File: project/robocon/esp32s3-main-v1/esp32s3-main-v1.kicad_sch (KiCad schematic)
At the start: 1 part, among them U1 ESP32-S3-WROOM-1

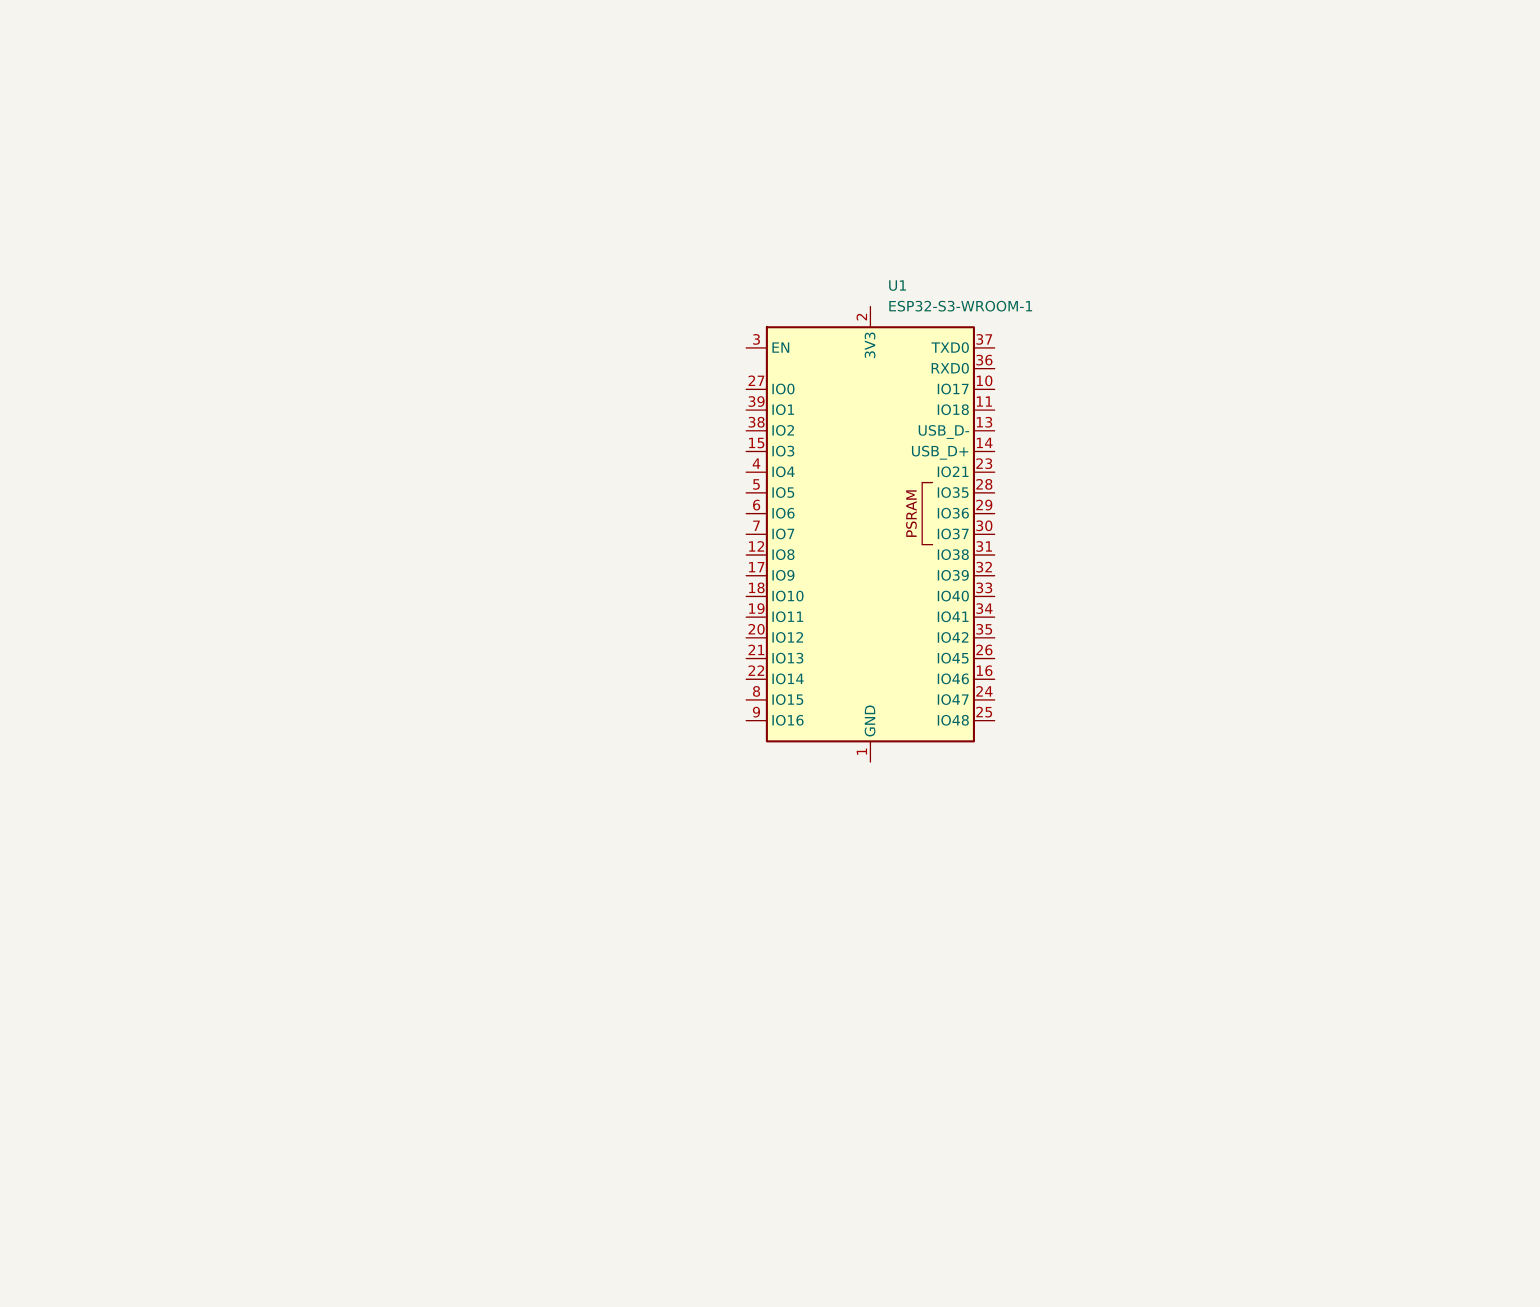
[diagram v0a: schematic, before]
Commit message: 2026/07/16/09:30
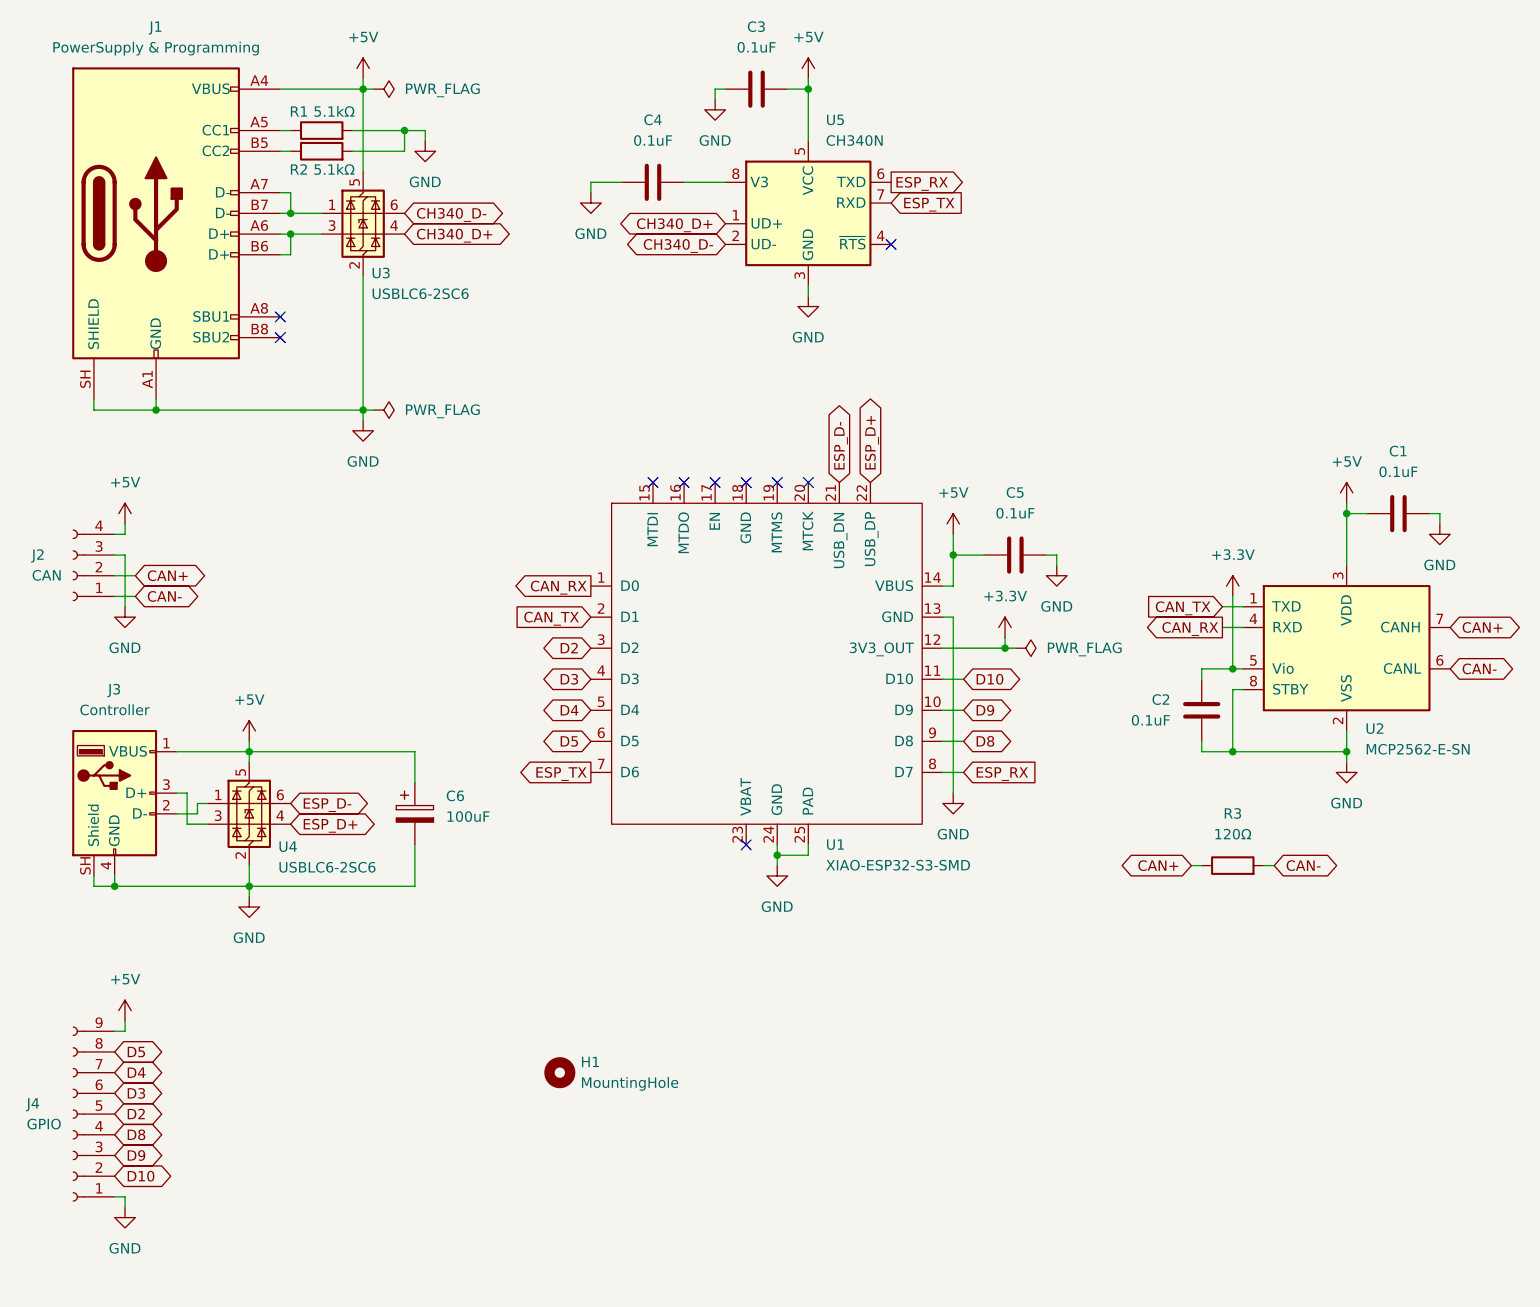
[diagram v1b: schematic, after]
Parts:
- removed U1: ESP32-S3-WROOM-1, RF_Module:ESP32-S3-WROOM-1, symbol RF_Module:ESP32-S3-WROOM-1
- added C1, C2, C3, C4, C5: 0.1uF, Capacitor_SMD:C_0603_1608Metric, symbol Device:C
- added C6: 100uF, Capacitor_THT:CP_Radial_D6.3mm_P2.50mm, symbol Device:C_Polarized
- added H1: MountingHole, MountingHole:MountingHole_3.2mm_M3, symbol Mechanical:MountingHole
- added J1: PowerSupply & Programming, Connector_USB:USB_C_Receptacle_GCT_USB4105-xx-A_16P_TopMnt_Horizontal, symbol Connector:USB_C_Receptacle_USB2.0_16P
- added J2: CAN, Connector_JST:JST_XH_S4B-XH-A_1x04_P2.50mm_Horizontal, symbol Connector:Conn_01x04_Socket
- added J3: Controller, Connector_USB:USB_A_Molex_67643_Horizontal, symbol Connector:USB_A
- added J4: GPIO, Connector_JST:JST_XH_B9B-XH-A_1x09_P2.50mm_Vertical, symbol Connector:Conn_01x09_Socket
- added R1, R2: 5.1kΩ, Resistor_SMD:R_0603_1608Metric, symbol Device:R
- added R3: 120Ω, Resistor_SMD:R_0603_1608Metric, symbol Device:R
- added U1: XIAO-ESP32-S3-SMD, Seeed Studio XIAO Series Library:XIAO-ESP32-S3-SMD, symbol Seeed_Studio_XIAO_Series:XIAO-ESP32-S3-SMD
- added U2: MCP2562-E-SN, Package_SO:SOIC-8_3.9x4.9mm_P1.27mm, symbol Interface_CAN_LIN:MCP2562-E-SN
- added U3, U4: USBLC6-2SC6, Package_TO_SOT_SMD:SOT-23-6, symbol Power_Protection:USBLC6-2SC6
- added U5: CH340N, Package_SO:JEITA_SOIC-8_3.9x4.9mm_P1.27mm, symbol Interface_USB:CH340N
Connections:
- new net: C4.1, U5.8 (V3)
- new net: J1.B5 (CC2), R2.1
- new net: J1.A5 (CC1), R1.1
- new net: J1.A7 (D-), J1.B7 (D-), U3.1 (I/O1)
- new net: J1.A6 (D+), J1.B6 (D+), U3.3 (I/O2)
- new net: J3.2 (D-), U4.1 (I/O1)
- new net: J3.3 (D+), U4.3 (I/O2)
- new net +3.3V: C2.1, U1.12 (3V3_OUT), U2.5 (Vio)
- new net +5V: C1.1, C3.1, C5.1, C6.1, J1.A4 (VBUS), J1.A9 (VBUS), J1.B4 (VBUS), J1.B9 (VBUS), J2.4 (Pin_4), J3.1 (VBUS), J4.9 (Pin_9), U1.14 (VBUS), U2.3 (VDD), U3.5 (VBUS), U4.5 (VBUS), U5.5 (VCC)
- new net CAN+: J2.2 (Pin_2), R3.1, U2.7 (CANH)
- new net CAN-: J2.1 (Pin_1), R3.2, U2.6 (CANL)
- new net CAN_RX: U1.1 (D0), U2.4 (RXD)
- new net CAN_TX: U1.2 (D1), U2.1 (TXD)
- new net CH340_D+: U3.4 (I/O2), U5.1 (UD+)
- new net CH340_D-: U3.6 (I/O1), U5.2 (UD-)
- new net D10: J4.2 (Pin_2), U1.11 (D10)
- new net D2: J4.5 (Pin_5), U1.3 (D2)
- new net D3: J4.6 (Pin_6), U1.4 (D3)
- new net D4: J4.7 (Pin_7), U1.5 (D4)
- new net D5: J4.8 (Pin_8), U1.6 (D5)
- new net D8: J4.4 (Pin_4), U1.9 (D8)
- new net D9: J4.3 (Pin_3), U1.10 (D9)
- new net ESP_D+: U1.22 (USB_DP), U4.4 (I/O2)
- new net ESP_D-: U1.21 (USB_DN), U4.6 (I/O1)
- new net ESP_RX: U1.8 (D7), U5.6 (TXD)
- new net ESP_TX: U1.7 (D6), U5.7 (RXD)
- new net GND: C1.2, C2.2, C3.2, C4.2, C5.2, C6.2, J1.A1 (GND), J1.A12 (GND), J1.B1 (GND), J1.B12 (GND), J1.SH (SHIELD), J2.3 (Pin_3), J3.4 (GND), J3.SH (Shield), J4.1 (Pin_1), R1.2, R2.2, U1.13 (GND), U1.24 (GND), U1.25 (PAD), U2.2 (VSS), U2.8 (STBY), U3.2 (GND), U4.2 (GND), U5.3 (GND)
- no-connect marks 0 -> 10

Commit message: 2026/07/16/16:32
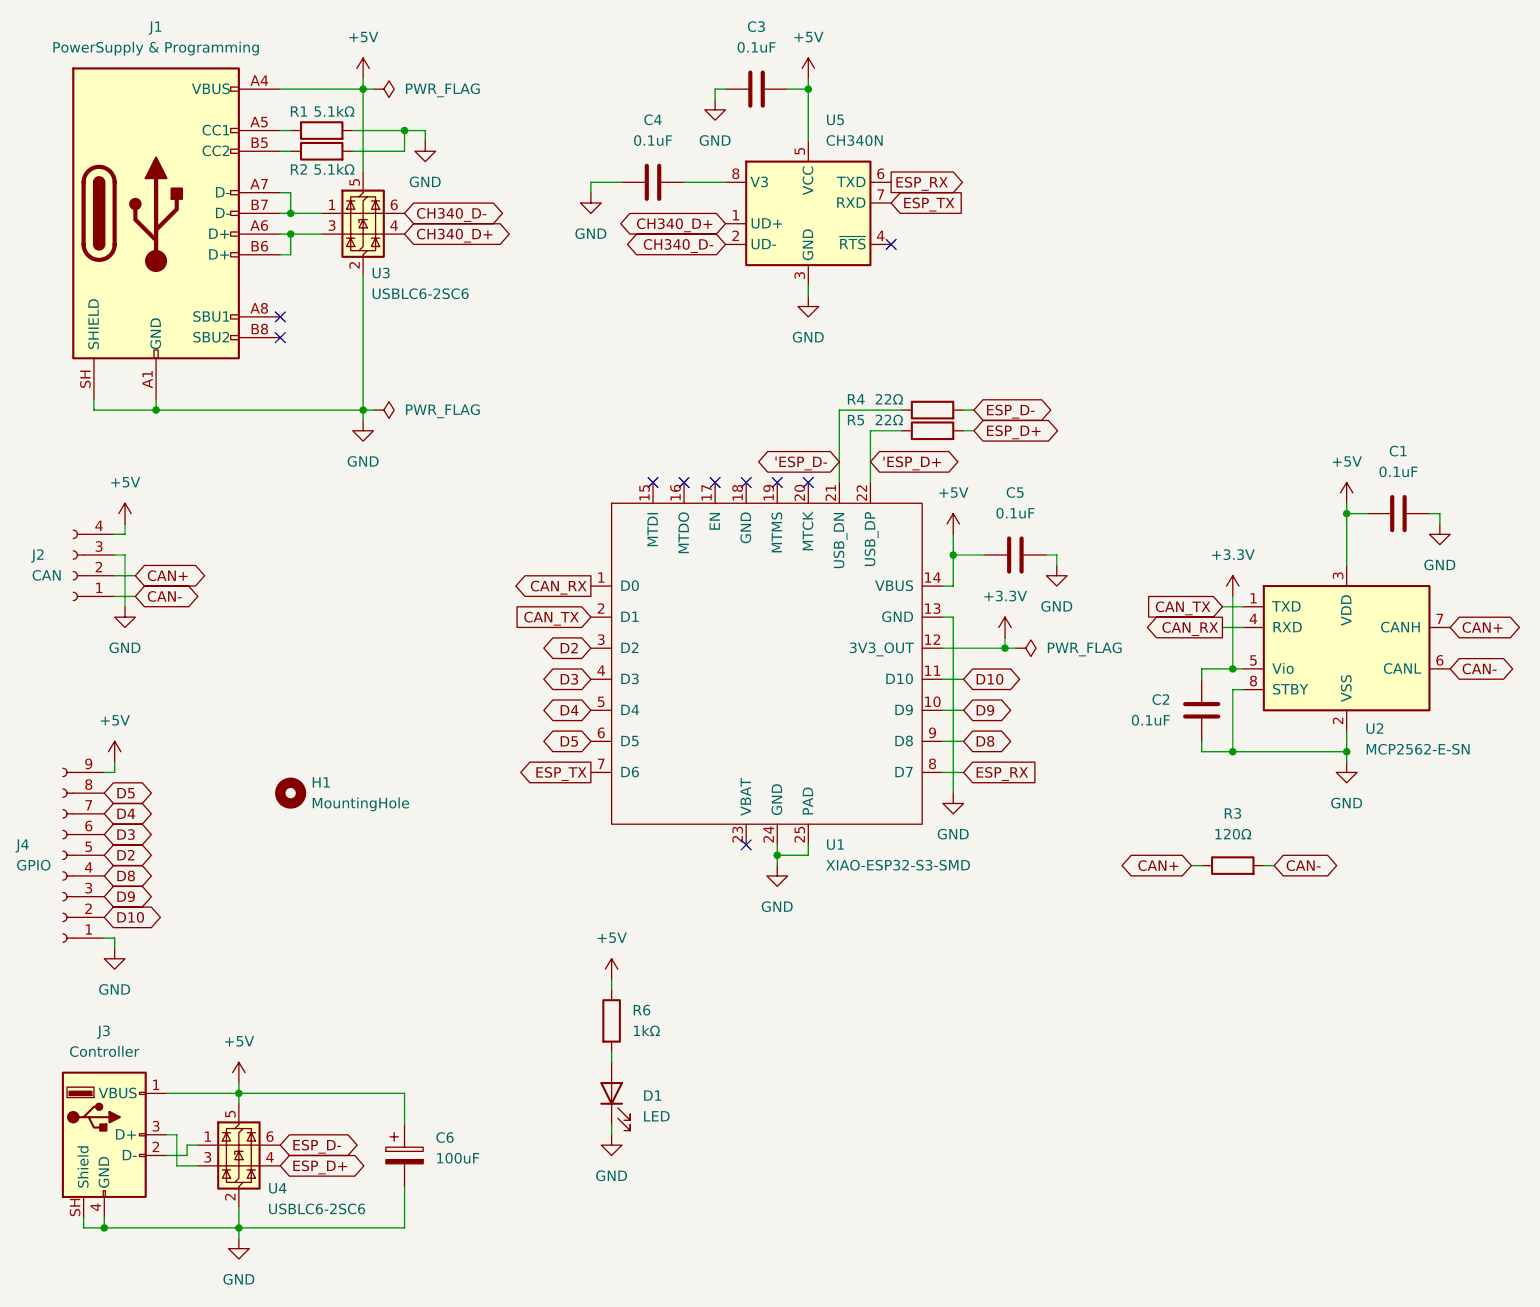
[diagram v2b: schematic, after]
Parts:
- added D1: LED, LED_SMD:LED_0603_1608Metric, symbol Device:LED
- added R4, R5: 22Ω, Resistor_SMD:R_0603_1608Metric, symbol Device:R
- added R6: 1kΩ, Resistor_SMD:R_0603_1608Metric, symbol Device:R
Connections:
- net +5V: now also R6.1
- net ESP_D+: now also R5.2; no longer U1.22 (USB_DP)
- net ESP_D-: now also R4.2; no longer U1.21 (USB_DN)
- net GND: now also D1.1 (K)
- new net: D1.2 (A), R6.2
- new net 'ESP_D+: R5.1, U1.22 (USB_DP)
- new net 'ESP_D-: R4.1, U1.21 (USB_DN)
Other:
- moved on the sheet: C6, H1, J3, J4, U4
